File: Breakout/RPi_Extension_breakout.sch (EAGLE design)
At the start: 7 parts

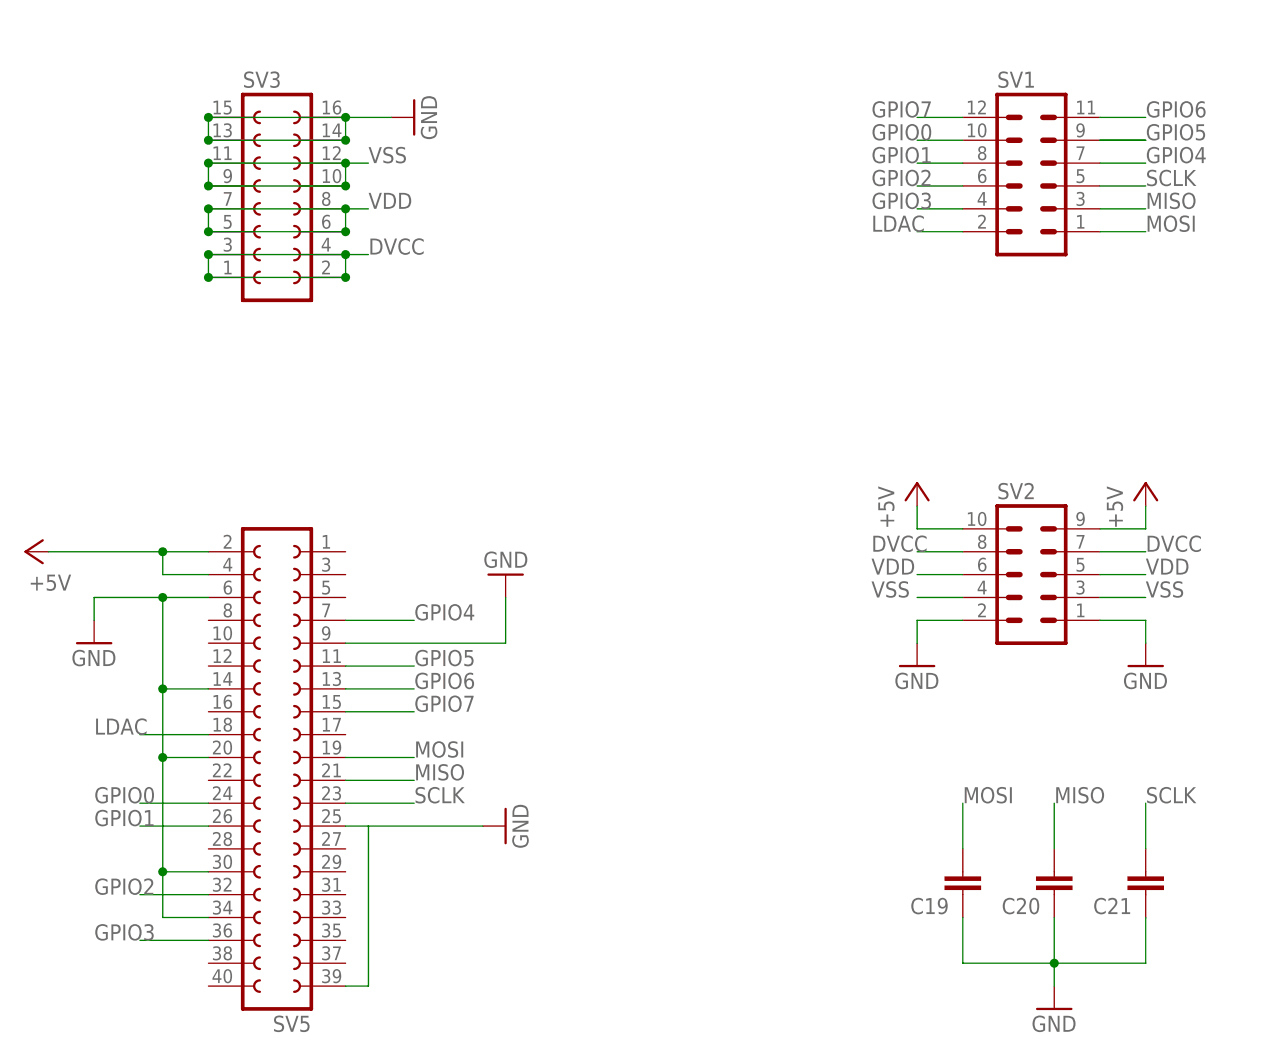
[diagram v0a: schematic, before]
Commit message: update
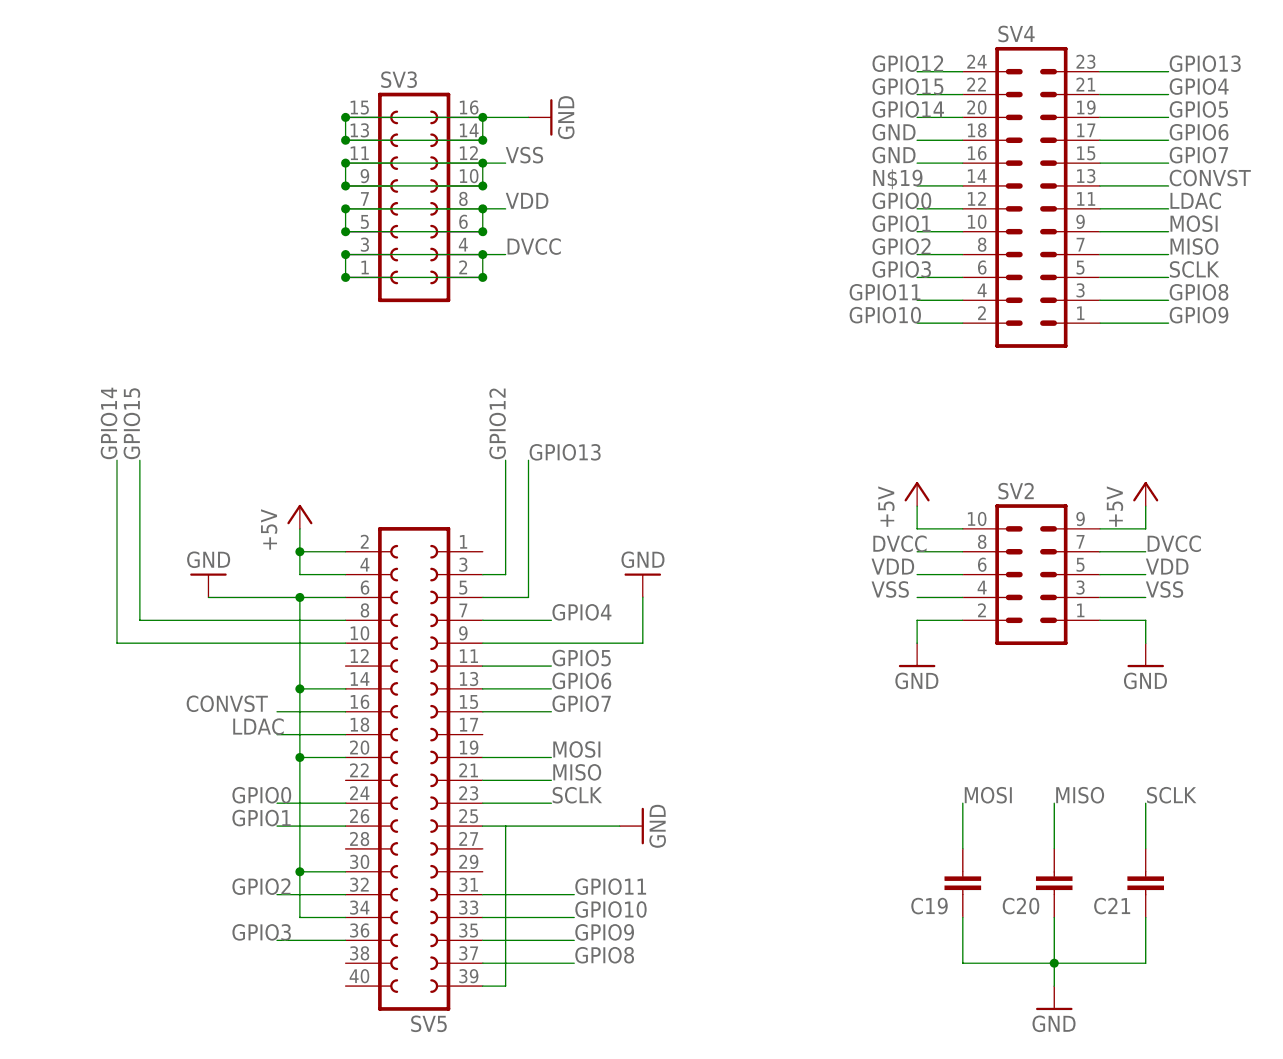
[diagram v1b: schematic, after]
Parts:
- removed SV1: (no value), con-lstb:MA06-2
- added SV4: (no value), con-lstb:MA12-2
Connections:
- new net CONVST: SV4.13, SV5.16
- new net GPIO10: SV4.2, SV5.33
- new net GPIO11: SV4.4, SV5.31
- new net GPIO12: SV4.24, SV5.3
- new net GPIO13: SV4.23, SV5.5
- new net GPIO14: SV4.20, SV5.10
- new net GPIO15: SV4.22, SV5.8
- new net GPIO8: SV4.3, SV5.37
- new net GPIO9: SV4.1, SV5.35
- new net N$19: SV4.14
- net GND: now also SV4.16, SV4.18
- net GPIO0: now also SV4.12; no longer SV1.10
- net GPIO1: now also SV4.10; no longer SV1.8
- net GPIO2: now also SV4.8; no longer SV1.6
- net GPIO3: now also SV4.6; no longer SV1.4
- net GPIO4: now also SV4.21; no longer SV1.7
- net GPIO5: now also SV4.19; no longer SV1.9
- net GPIO6: now also SV4.17; no longer SV1.11
- net GPIO7: now also SV4.15; no longer SV1.12
- net LDAC: now also SV4.11; no longer SV1.2
- net MISO: now also SV4.7; no longer SV1.3
- net MOSI: now also SV4.9; no longer SV1.1
- net SCLK: now also SV4.5; no longer SV1.5
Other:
- moved on the sheet: SV3, SV5
